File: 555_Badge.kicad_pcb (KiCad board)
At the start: 2 copper layers, 15 parts, among them Q1 2N3904

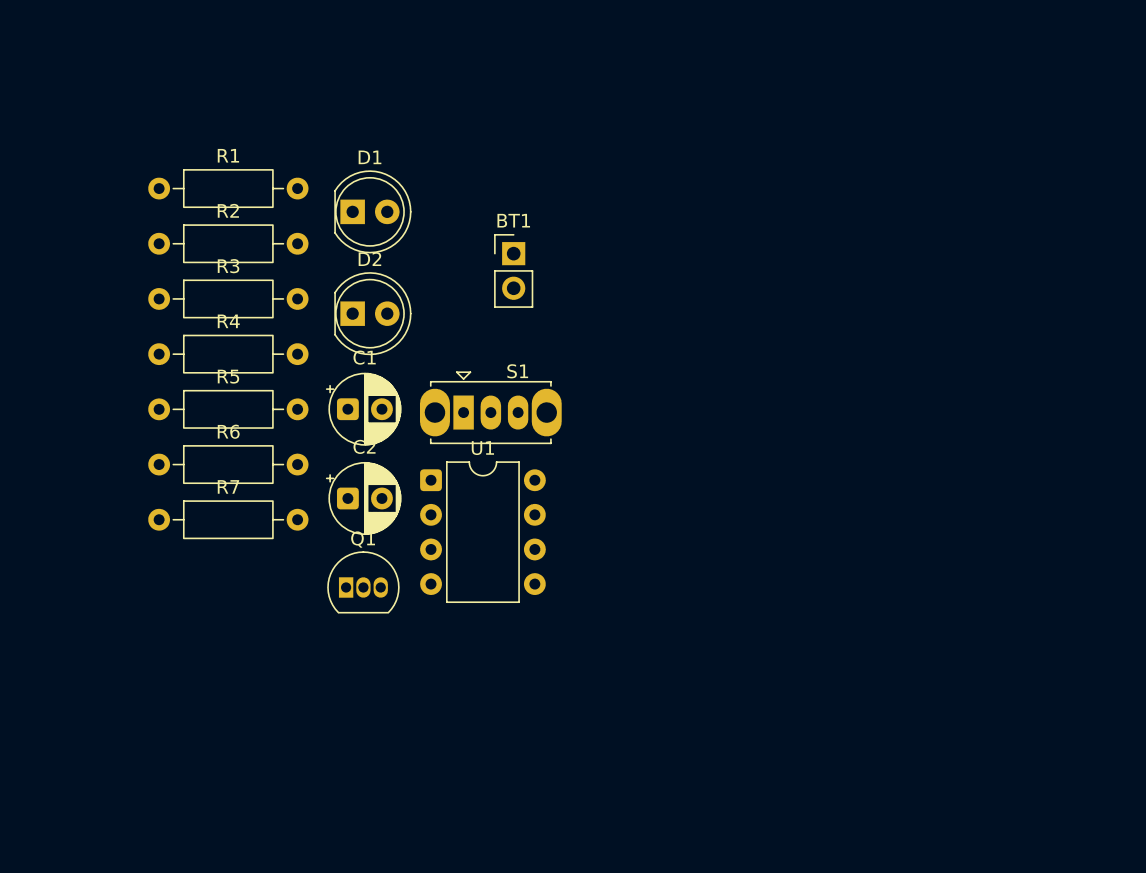
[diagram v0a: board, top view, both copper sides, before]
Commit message: Add completed PCB layout and gerber files
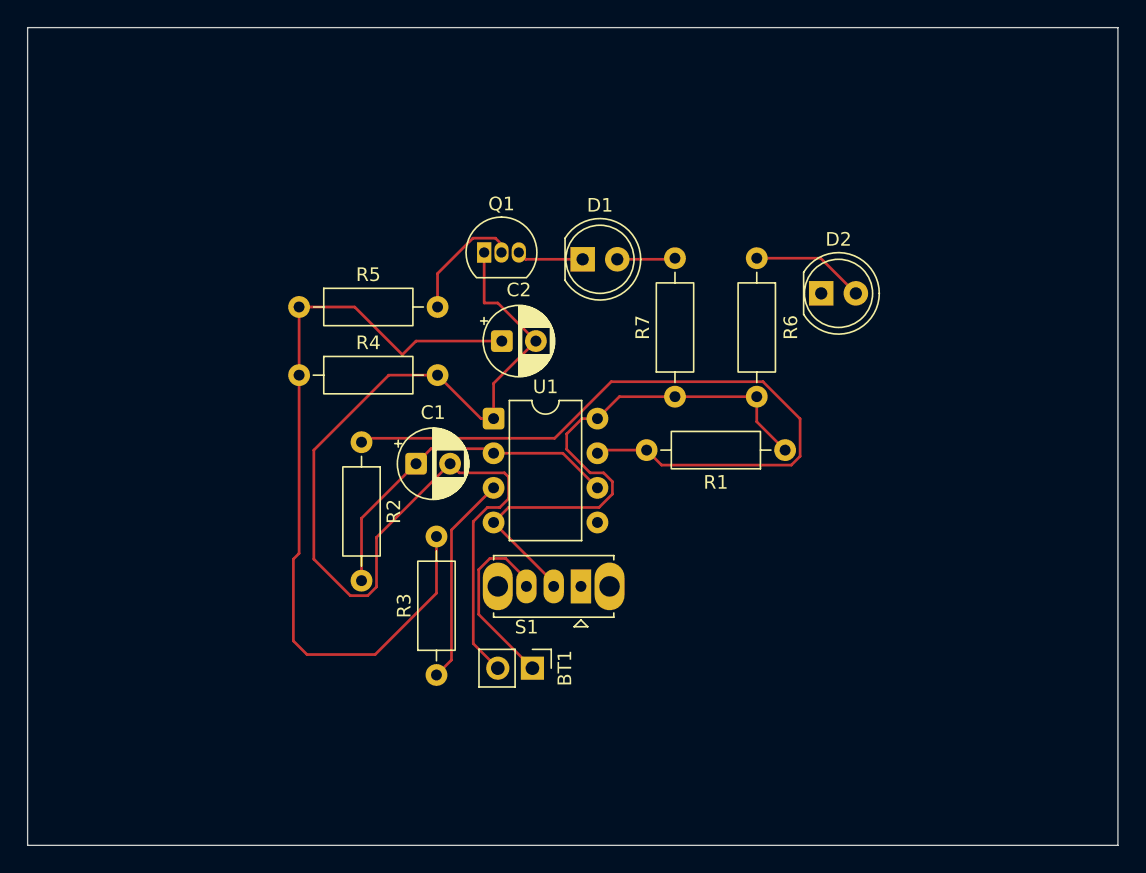
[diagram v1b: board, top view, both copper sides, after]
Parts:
- R1: value 22K -> 4.7K
- R2: value 330K -> 68K
- R6, R7: value 100 -> 470
- moved R1 49.8 mm to (67.6, 43.0), turned to 180 degrees
- moved R6 46.4 mm to (65.5, 28.9), turned to -90 degrees
- moved R7 38.9 mm to (59.5, 39.1), turned to 90 degrees
- moved D2 34.4 mm to (70.2, 31.5)
- moved R3 34.3 mm to (42.0, 59.5), turned to 90 degrees
- moved BT1 30.4 mm to (49.0, 59.0), turned to -90 degrees
- moved Q1 26.6 mm to (45.5, 28.5)
- moved R2 20.8 mm to (36.5, 42.4), turned to -90 degrees
- moved D1 17.2 mm to (52.7, 29.0)
- moved C2 16.2 mm to (46.8, 35.0)
- moved S1 15.4 mm to (52.6, 53.0), turned to 180 degrees
- moved R5 12.7 mm to (31.9, 32.5)
- moved R4 10.4 mm to (31.9, 37.5)
- moved U1 6.44 mm to (46.2, 40.7)
- moved C1 6.40 mm to (40.5, 44.0)
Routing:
- net GND: track 0.00 -> 78.7 mm
- net Net-(C2-Pad1): track 0.00 -> 58.4 mm
- net Net-(U1-DIS): track 0.00 -> 53.6 mm
- net VCC: track 0.00 -> 42.3 mm
- net Net-(U1-THRESH): track 0.00 -> 25.2 mm
- net Net-(U1-OUT): track 0.00 -> 15.5 mm
- net Net-(BT1-+): track 0.00 -> 13.9 mm
- net Net-(Q1-B): track 0.00 -> 9.01 mm
- net Net-(D2-A): track 0.00 -> 8.34 mm
- net Net-(D1-K): track 0.00 -> 4.89 mm
- net Net-(D1-A): track 0.00 -> 4.27 mm
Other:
- board outline added: 80 x 60 mm
